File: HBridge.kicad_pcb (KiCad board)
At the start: 2 copper layers, 29 x 28 mm, 28 parts, among them Q1 DMG2301L, Q2 DMG3402L, Q3 DMG2301L, Q4 DMG3402L, U1 74LVC1GU04DRL, U10 LT1762, U2 74AHC1G08, U3 74AHC1G08, U4 74AHC1G08, U5 74AHC1G08, U6 74LVC1GU04DRL, U7 74LVC1GU04DRL, U8 74LVC1GU04DRL

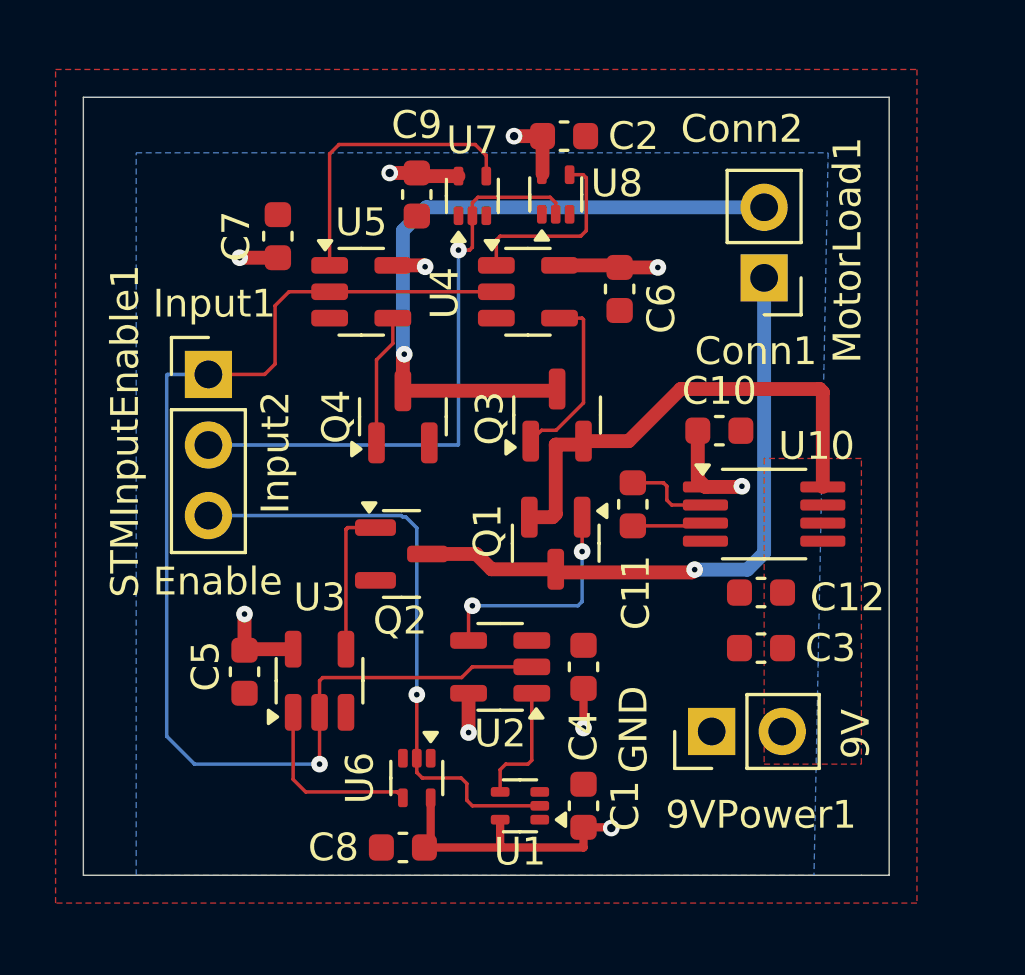
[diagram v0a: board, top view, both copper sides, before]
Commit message: layout and routing version 2
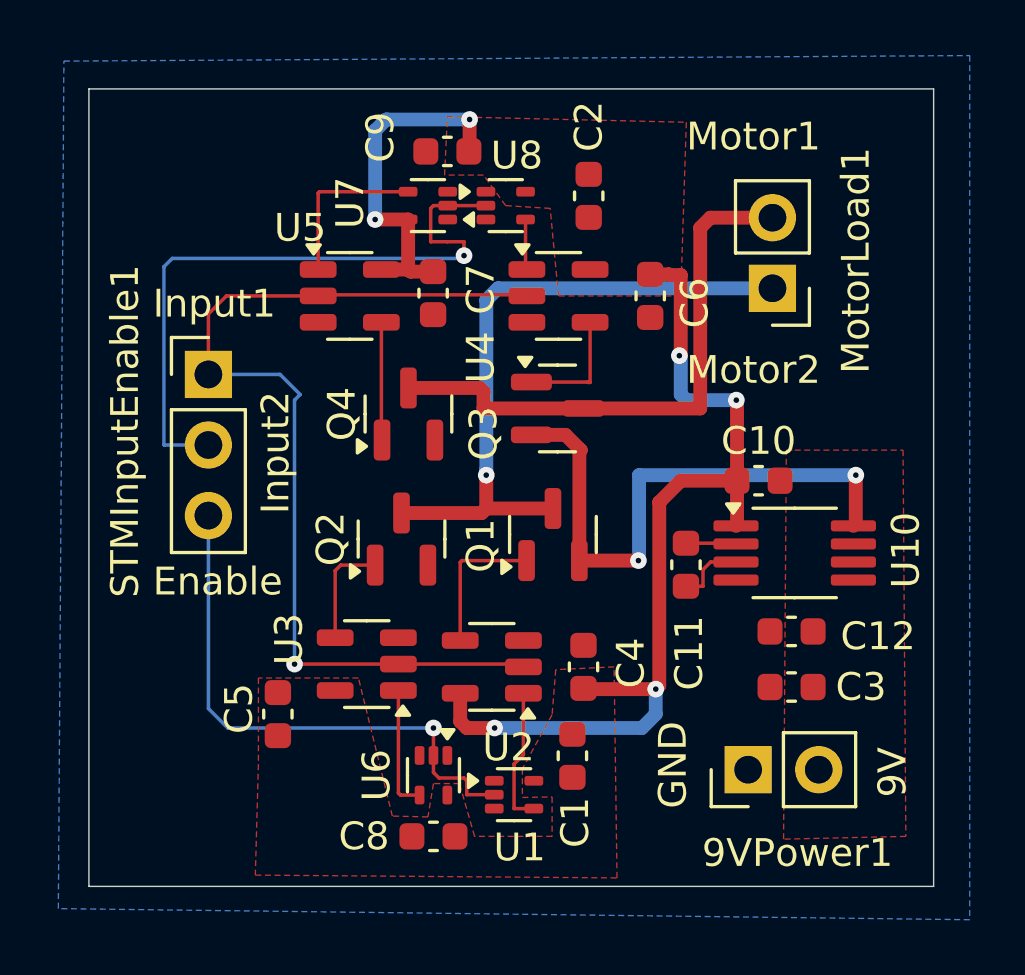
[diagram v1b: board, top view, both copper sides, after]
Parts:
- moved C7 5.95 mm to (181.6, 75.0), turned to -90 degrees
- moved C11 2.90 mm to (190.7, 84.8)
- moved C2 2.33 mm to (187.2, 71.5), turned to 90 degrees
- moved C10 2.29 mm to (193.3, 81.8)
- moved C5 1.94 mm to (176.0, 90.2)
- moved 9VPower1 1.90 mm to (192.9, 92.2)
- moved C9 1.90 mm to (182.1, 70.0), turned to 180 degrees
- moved U8 1.84 mm to (184.2, 71.9), turned to 0 degrees
- moved C1 1.84 mm to (186.6, 91.7)
- moved U3 1.80 mm to (179.2, 88.4), turned to 180 degrees
- moved C12 1.78 mm to (194.5, 87.2)
- moved C3 1.78 mm to (194.5, 89.2)
- moved U10 1.78 mm to (194.6, 84.4)
- moved U7 1.64 mm to (181.4, 71.9), turned to 180 degrees
- moved C8 1.17 mm to (181.6, 94.6)
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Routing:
- net +3.3V: track 31.0 -> 46.9 mm, vias 10 -> 6
- net /Enable: track 44.1 -> 35.6 mm
- net Net-(U4-Pad1): track 6.84 -> 1.82 mm
- net Net-(U5-Pad1): track 10.7 -> 6.01 mm
- net /MotorConnect1: track 24.8 -> 20.4 mm, vias 1 -> 0
- net +9V: track 17.4 -> 20.7 mm, vias 0 -> 2
- net Net-(Q1-G): track 8.43 -> 5.23 mm, vias 2 -> 0
- net Net-(U3-Pad1): track 6.64 -> 4.48 mm
- net Net-(Q3-G): track 6.35 -> 4.28 mm
- net /Input1: track 21.8 -> 19.7 mm
- net /Input2: track 22.1 -> 24.0 mm
- net Net-(Q2-G): track 5.47 -> 3.93 mm
- net Net-(U10-ADJ): track 3.24 -> 1.81 mm
- net /MotorConnect2: track 22.6 -> 23.5 mm
- net Net-(U1-Pad4): track 4.49 -> 5.00 mm
- added copper zone on F.Cu, net +3.3V
- added copper zone on B.Cu, net GND
- removed copper zone on B.Cu, net +3.3V
- removed copper zone on F.Cu, net GND
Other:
- board size 29 x 28 mm -> 30.4 x 28.7 mm
- board text added: "Motor1"
- board text added: "Motor2"
- board text removed: "Conn1"
- board text removed: "Conn2"
